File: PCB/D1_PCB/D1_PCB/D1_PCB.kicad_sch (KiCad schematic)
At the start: 39 parts, among them J1 BB_RIGHT, J2 BB_LEFT, J3 Conn_01x02, J4 Conn_01x02, J5 Conn_01x04_Pin, U1 WEMOS_D1_mini, t3v3 TestPoint, t5V1 TestPoint

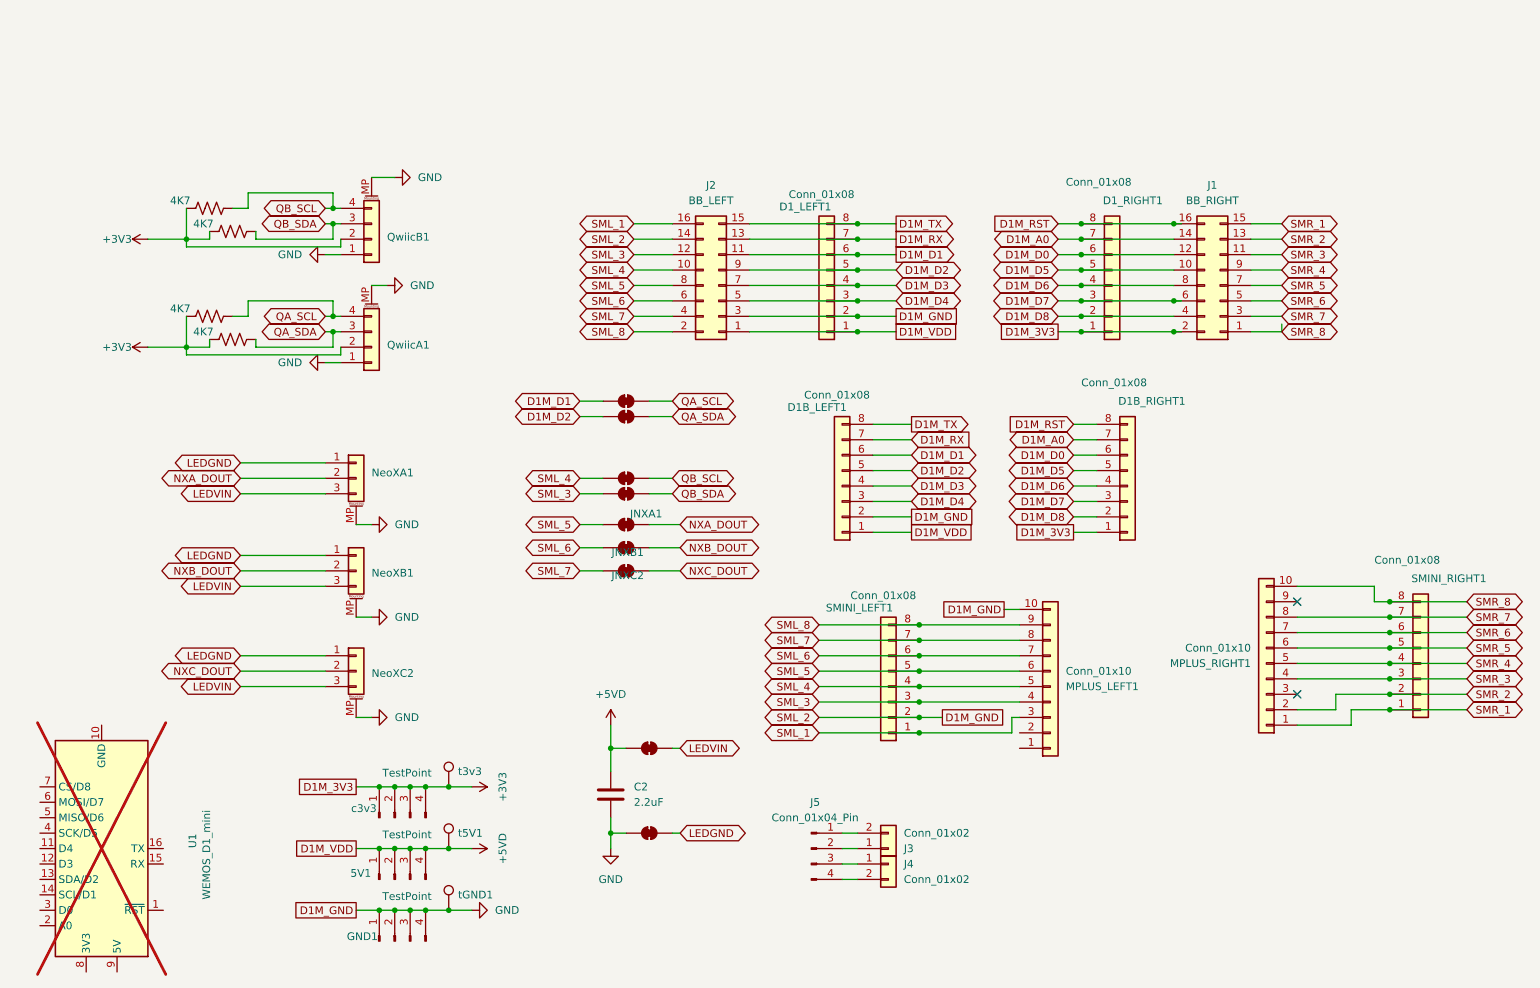
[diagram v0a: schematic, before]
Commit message: PCB changes
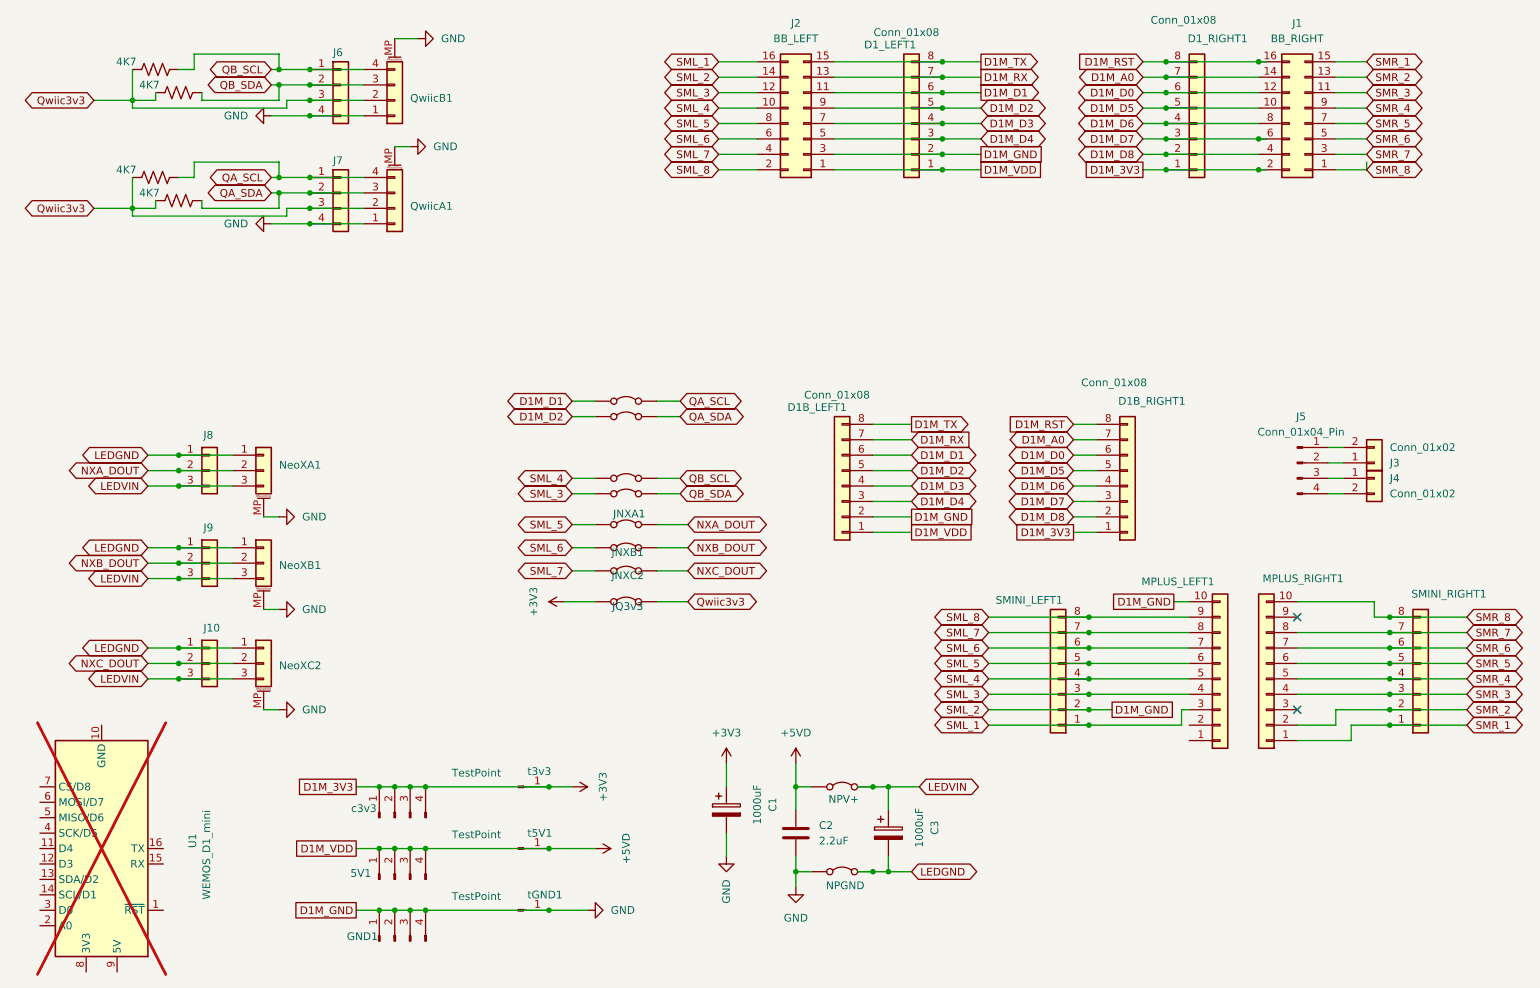
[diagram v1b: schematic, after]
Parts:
- added C1, C3: 1000uF, Capacitor_THT:CP_Radial_D4.0mm_P1.50mm, symbol Device:C_Polarized
- added J10, J8, J9: Conn_01x03, Connector_PinHeader_2.54mm:PinHeader_1x03_P2.54mm_Vertical, symbol Connector_Generic:Conn_01x03
- added J6, J7: Conn_01x04, Connector_PinHeader_2.54mm:PinHeader_1x04_P2.54mm_Vertical, symbol Connector_Generic:Conn_01x04
- added JQ3v3: SolderJumper_2_Bridged, Connector_PinHeader_2.54mm:PinHeader_1x02_P2.54mm_Vertical, symbol Jumper:Jumper_2_Bridged
- J1, J2: footprint Connector_PinHeader_2.54mm:PinHeader_2x08_P2.54mm_Vertical -> Connector_IDC:IDC-Header_2x08_P2.54mm_Vertical
- JLGND1: value SolderJumper_2_Bridged -> NPGND; footprint Jumper:SolderJumper-2_P1.3mm_Bridged2Bar_RoundedPad1.0x1.5mm -> Connector_PinHeader_2.54mm:PinHeader_1x02_P2.54mm_Vertical; symbol Jumper:SolderJumper_2_Bridged -> Jumper:Jumper_2_Bridged; now in the parts list
- JLVDD1: value SolderJumper_2_Bridged -> NPV+; footprint Jumper:SolderJumper-2_P1.3mm_Bridged2Bar_RoundedPad1.0x1.5mm -> Connector_PinHeader_2.54mm:PinHeader_1x02_P2.54mm_Vertical; symbol Jumper:SolderJumper_2_Bridged -> Jumper:Jumper_2_Bridged; now in the parts list
- JNXA1, JNXB1, JNXC2, SCL_A1, SCL_B1, SDA_A1, SDA_B1: footprint Jumper:SolderJumper-2_P1.3mm_Bridged2Bar_RoundedPad1.0x1.5mm -> Connector_PinHeader_2.54mm:PinHeader_1x02_P2.54mm_Vertical; symbol Jumper:SolderJumper_2_Bridged -> Jumper:Jumper_2_Bridged; now in the parts list
- t3v3, t5V1, tGND1: footprint Connector_Pin:Pin_D1.3mm_L11.0mm -> Connector_PinHeader_2.54mm:PinHeader_1x01_P2.54mm_Vertical; symbol Connector:TestPoint -> Connector:Conn_01x01_Pin
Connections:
- net +3V3: now also C1.1, JQ3v3.1 (A); no longer QwiicA1.2 (Pin_2), QwiicB1.2 (Pin_2), R1.1, R2.1, R3.1, R4.1
- net GND: now also C1.2, J6.4 (Pin_4), J7.4 (Pin_4)
- net LEDGND: now also C3.2, J10.1 (Pin_1), J8.1 (Pin_1), J9.1 (Pin_1)
- net LEDVIN: now also C3.1, J10.3 (Pin_3), J8.3 (Pin_3), J9.3 (Pin_3)
- net NXA_DOUT: now also J8.2 (Pin_2)
- net NXB_DOUT: now also J9.2 (Pin_2)
- net NXC_DOUT: now also J10.2 (Pin_2)
- net QA_SCL: now also J7.1 (Pin_1)
- net QA_SDA: now also J7.2 (Pin_2)
- net QB_SCL: now also J6.1 (Pin_1)
- net QB_SDA: now also J6.2 (Pin_2)
- new net Qwiic3v3: J6.3 (Pin_3), J7.3 (Pin_3), JQ3v3.2 (B), QwiicA1.2 (Pin_2), QwiicB1.2 (Pin_2), R1.1, R2.1, R3.1, R4.1
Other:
- moved on the sheet: C2, D1_LEFT1, D1_RIGHT1, J1, J2, J3, J4, J5, MPLUS_LEFT1, MPLUS_RIGHT1, NeoXA1, NeoXB1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
